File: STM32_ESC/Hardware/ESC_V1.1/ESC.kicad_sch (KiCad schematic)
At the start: 91 parts, among them IC1 IR2103STRPBF, IC2 LMR51420XDDCR, IC3 IR2103STRPBF, IC4 IR2103STRPBF, J1 USB_C_Receptacle_USB2.0_16P, Q1 BSC060P03NS3E G, Q2 BSC060P03NS3E G, Q3 BSC060P03NS3E G, Q4 BSC060P03NS3E G, Q5 IRFH8318TRPBF, Q6 BSC060P03NS3E G, Q7 BSC060P03NS3E G, U1 STM32L412CBU6, U2 USBLC6-2SC6, U3 INA180A3, U4 INA180A3, U5 INA180A3, Y1 Crystal_GND24_Small

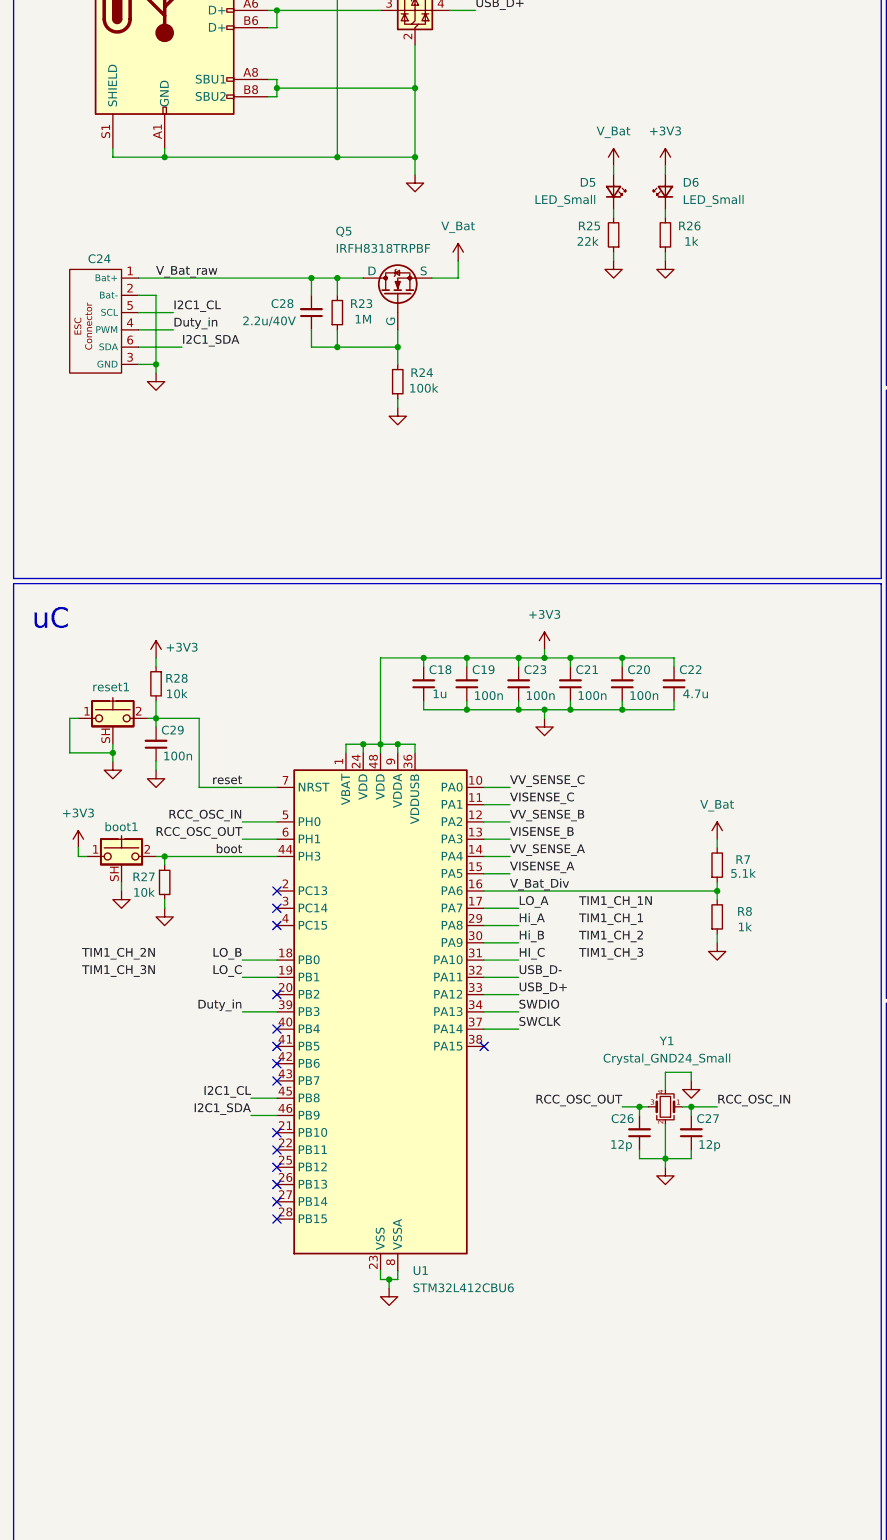
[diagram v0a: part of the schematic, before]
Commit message: updated
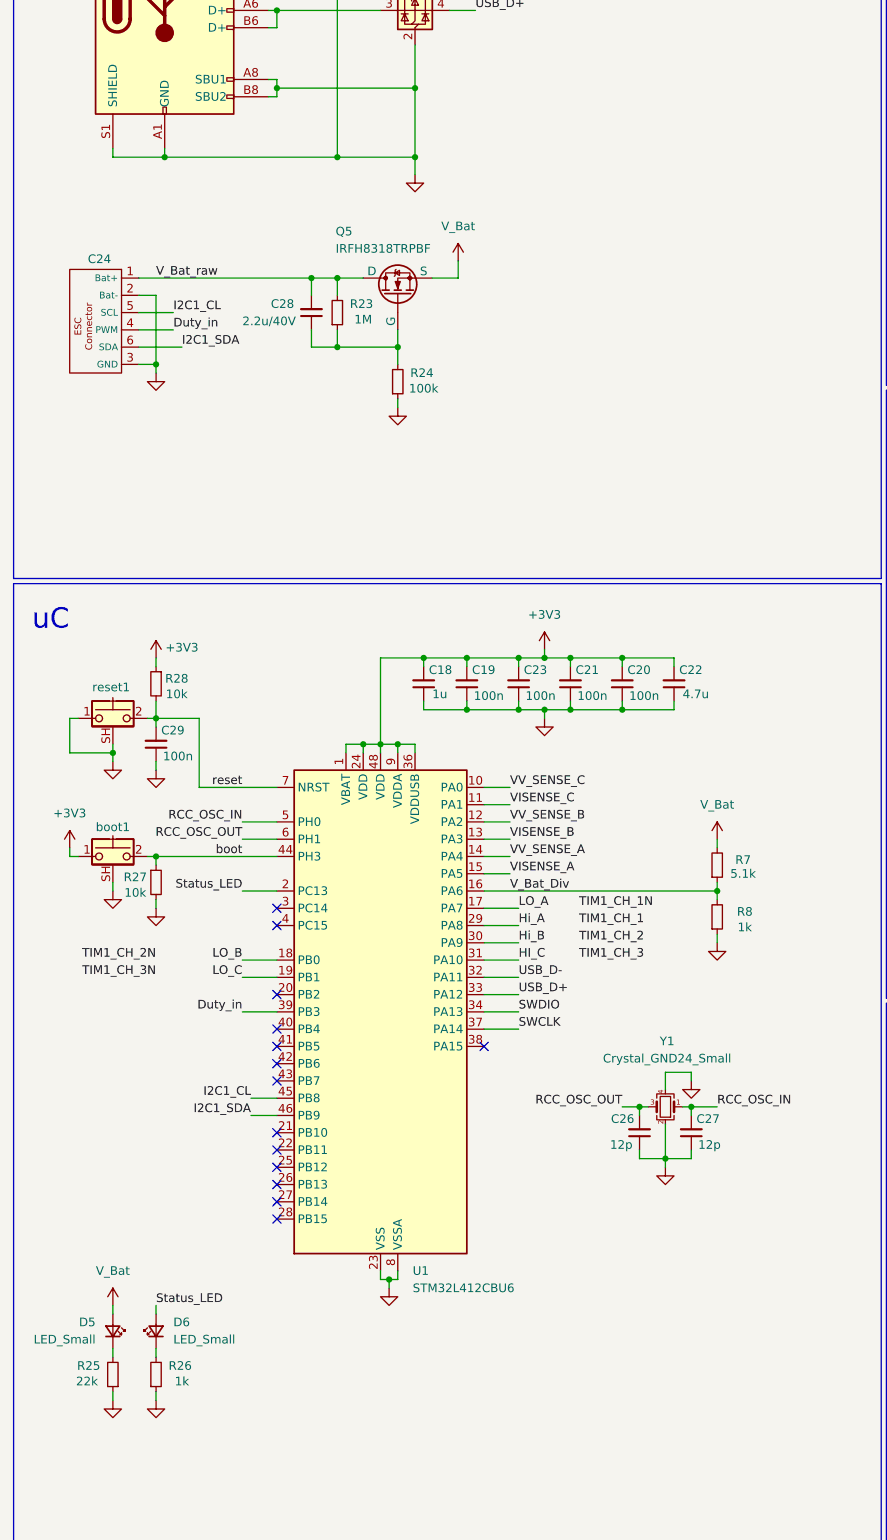
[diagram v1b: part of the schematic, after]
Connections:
- net +3V3: no longer D6.2 (A)
- net Status_LED: now reaches U1.2 (PC13)
- net Status_LED: now also D6.2 (A)
- no-connect marks 15 -> 14
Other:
- moved on the sheet: D5, D6, R25, R26, R27, boot1
